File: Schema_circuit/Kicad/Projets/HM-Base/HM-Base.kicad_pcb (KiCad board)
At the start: 2 copper layers, 110 x 67 mm, 16 parts, among them J1A1 Conn_01x02_Socket, J2A1 Conn_01x02_Socket, J3A1 Conn_01x06_Socket, J4A1 Conn_01x06_Socket, J5A1 Conn_01x08_Socket, J6A1 Conn_01x02_Socket, U1 TP4056, U2 TPS63020, U3 ESP32-DEVKITC-32D

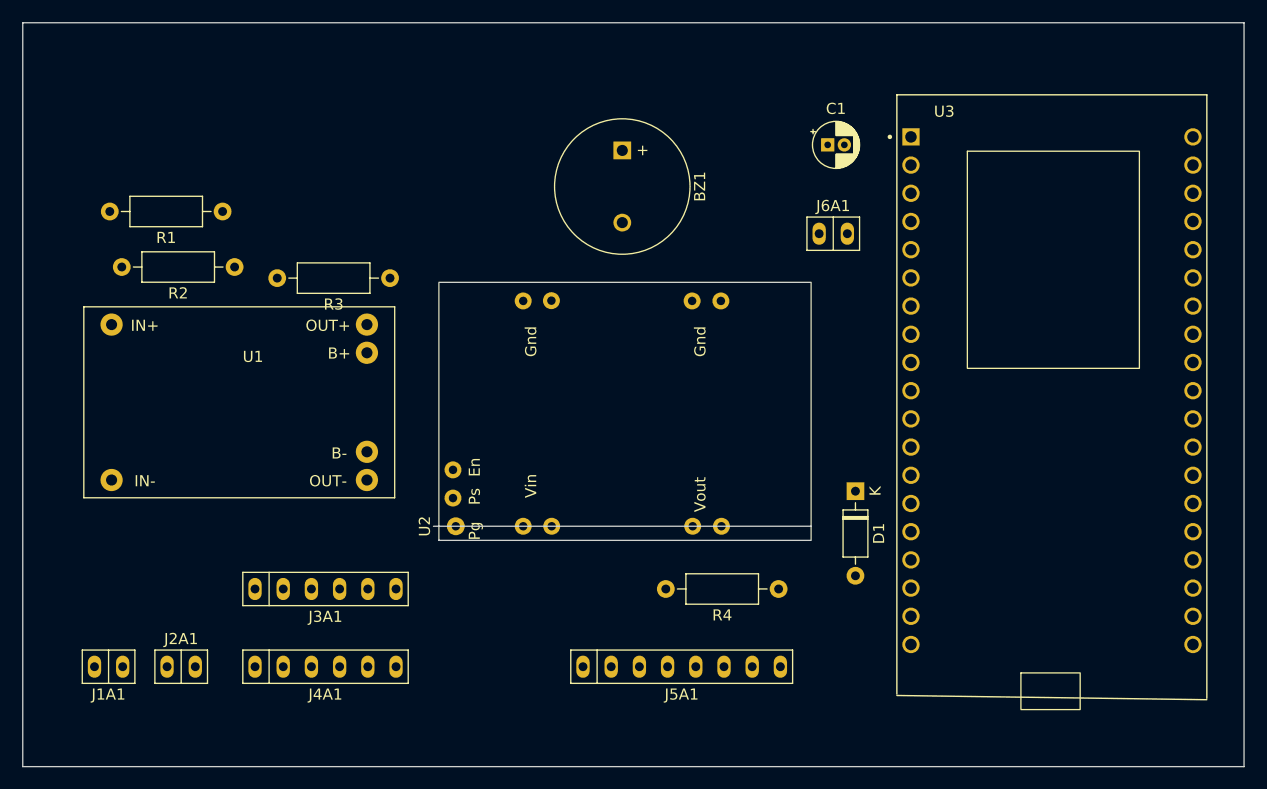
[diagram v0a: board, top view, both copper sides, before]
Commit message: Rectification schema BASE
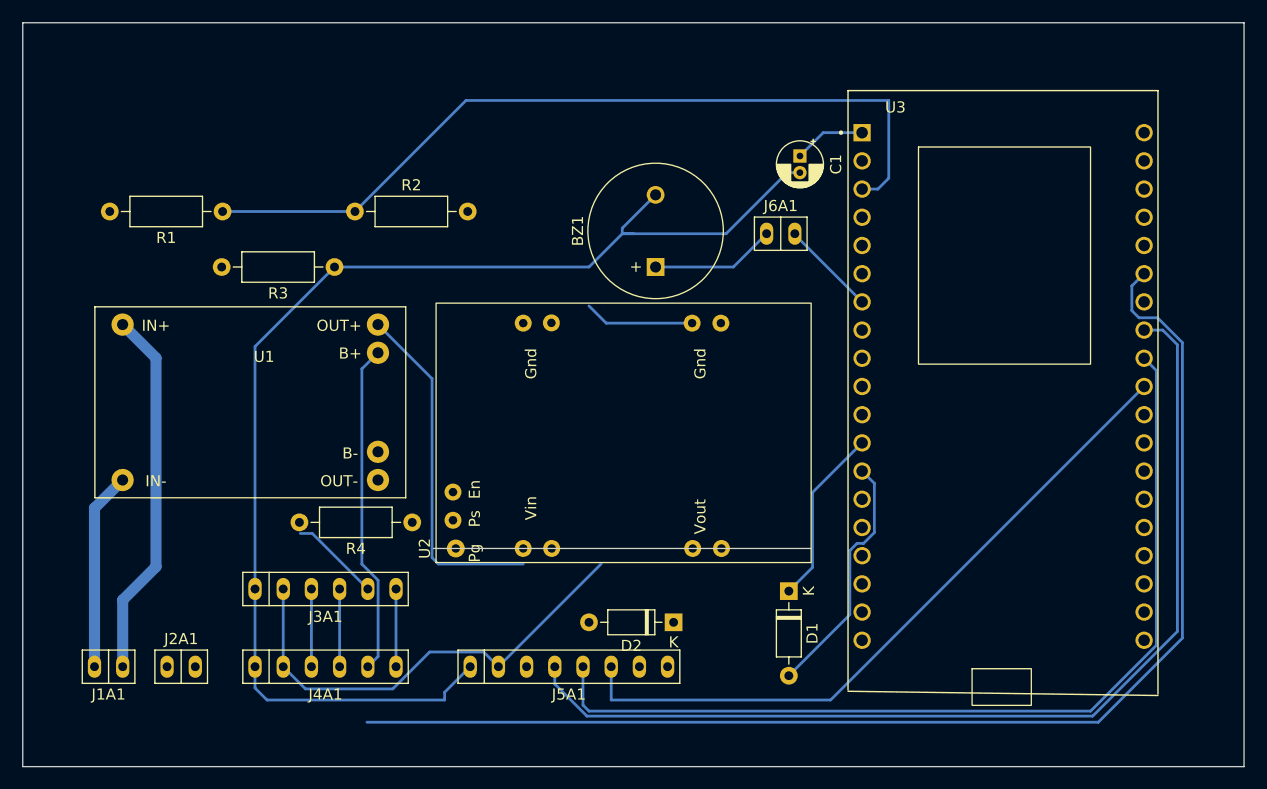
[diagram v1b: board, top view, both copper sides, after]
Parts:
- added D2: 1N4148, Diode_THT:D_DO-35_SOD27_P7.62mm_Horizontal, F.Cu at (139.6, 101.0)
- moved R4 33.5 mm to (116.1, 92.0)
- moved R2 11.9 mm to (110.9, 64.0), turned to 0 degrees
- moved BZ1 10.9 mm to (138.0, 69.0), turned to 90 degrees
- moved D1 10.8 mm to (150.0, 98.2)
- moved J5A1 10.2 mm to (130.2, 105.0)
- moved R3 5.10 mm to (109.1, 69.0)
- moved J6A1 4.73 mm to (149.3, 66.0)
- moved U3 4.42 mm to (169.3, 76.0)
- moved C1 2.69 mm to (151.0, 59.0), turned to -90 degrees
- moved U2 2.00 mm to (135.0, 94.4)
- moved U1 1.00 mm to (87.5, 89.8)
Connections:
- R4 pad 1: Net-(D1-K) -> Net-(J3A1-Pin_5)
- R4 pad 2: Net-(J3A1-Pin_5) -> Net-(D2-A)
- U3 pad J2-12: Net-(D1-K) -> Net-(D2-A)
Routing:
- net GND: track 0.00 -> 123.5 mm
- net /SDA: track 0.00 -> 119.7 mm
- net /MISO: track 0.00 -> 91.4 mm
- net /CLK: track 0.00 -> 84.1 mm
- net Net-(U3-SENSOR_VP): track 0.00 -> 73.9 mm
- net /CS: track 0.00 -> 62.7 mm
- net +3.3V: track 0.00 -> 48.7 mm
- net Net-(J1A1-Pin_2): track 0.00 -> 33.3 mm
- net Net-(U1-Vout1): track 0.00 -> 31.5 mm
- net Net-(J4A1-Pin_5): track 0.00 -> 29.9 mm
- net Net-(D1-A): track 0.00 -> 22.4 mm
- net Net-(J1A1-Pin_1): track 0.00 -> 17.9 mm
- net Net-(D1-K): track 0.00 -> 16.1 mm
- net Net-(BZ1--): track 0.00 -> 11.6 mm
- net Net-(J6A1-Pin_1): track 0.00 -> 8.65 mm
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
